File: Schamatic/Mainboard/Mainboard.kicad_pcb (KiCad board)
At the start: 2 copper layers, 45 x 130 mm, 277 parts, among them J1 CONN_01X02, J10 CONN_01X04, J2 CONN_01X02, J3 CONN_01X02, J4 CONN_01X02, J5 CONN_01X02, J6 CONN_02X05, J7 CONN_02X20, J8 CONN_01X02, J9 CONN_01X02, Q1 Q_NMOS_GDS, Q2 PSMN014-40YS, U1 LM2678-3.3V, U10 LTC2954, U2 LM2678-5V, U3 MC78M00, U4 LM5122, U5 UCC27611, U6 ACS781, U7 LSM6DS33, U8 STM32F031G6U6, U9 LTC2876, Y1 Resonator_Small

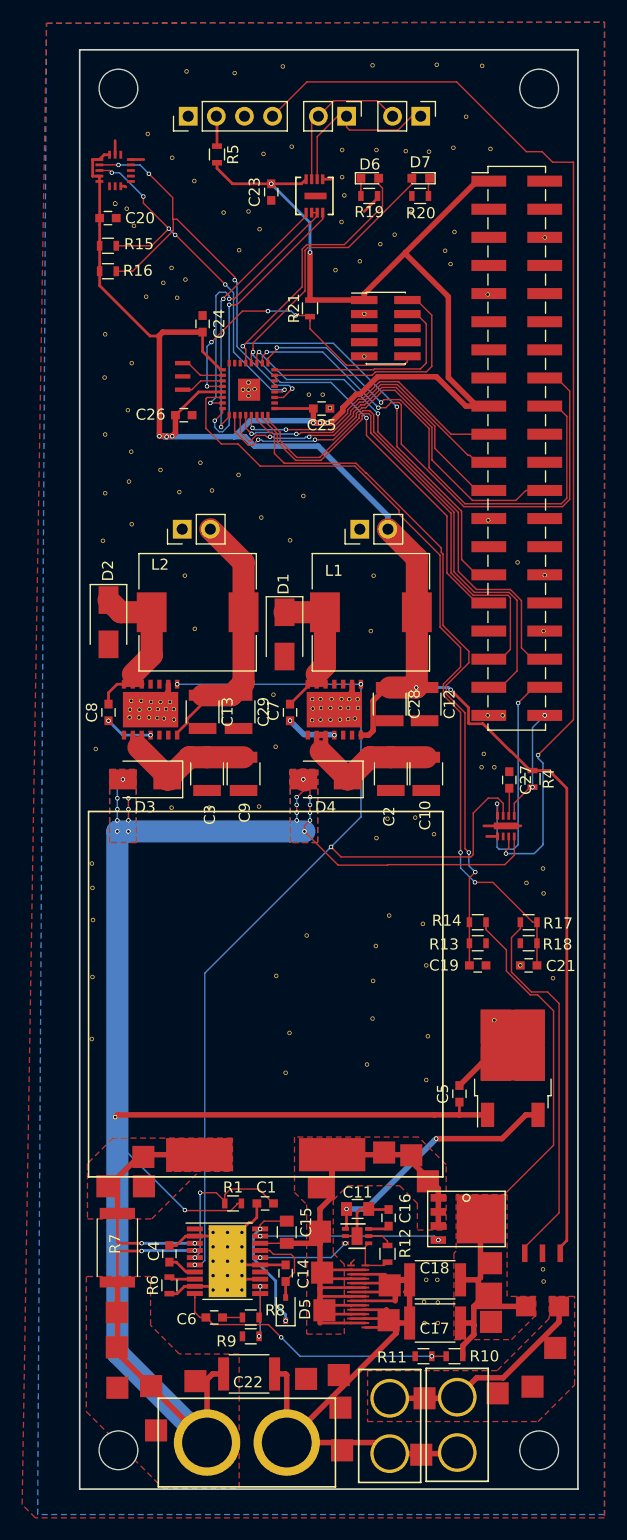
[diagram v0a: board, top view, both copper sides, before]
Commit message: changes
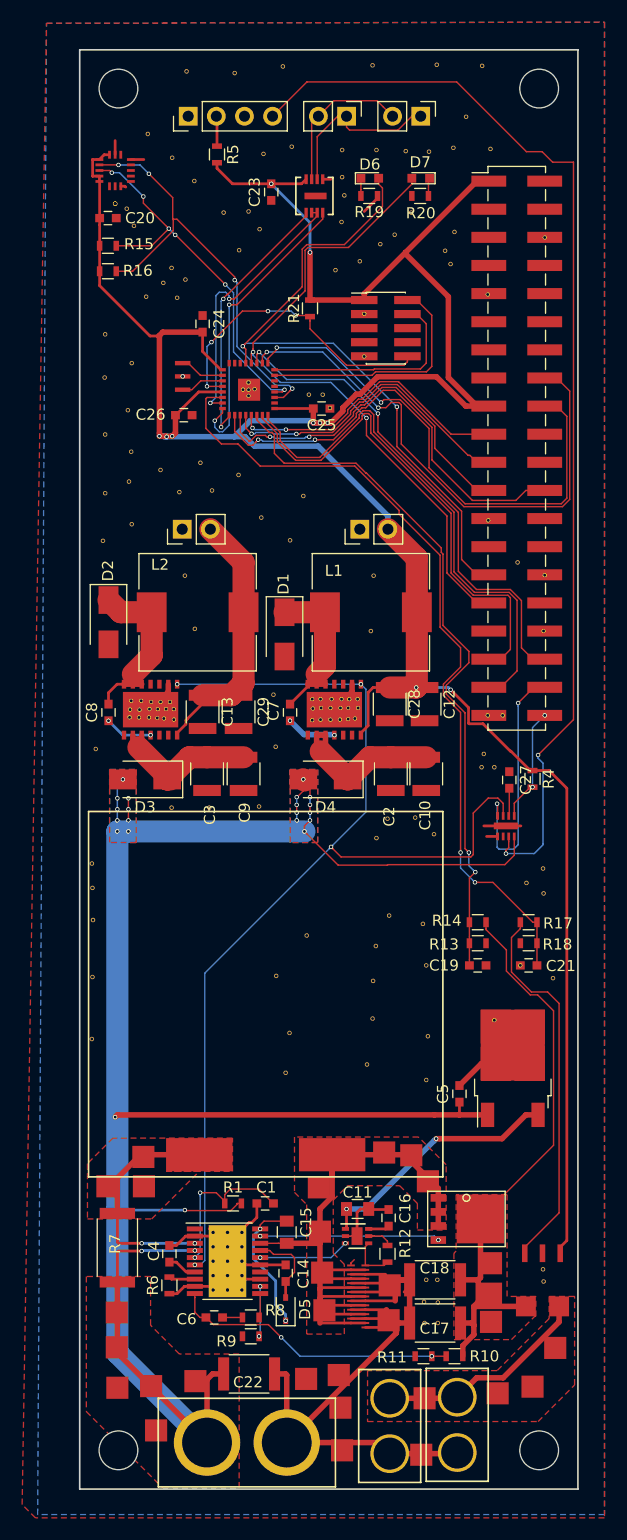
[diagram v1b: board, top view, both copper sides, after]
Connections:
- Y1 pad 2: (no net) -> Earth
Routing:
- net +BATT: track 200.3 -> 195.4 mm
- net 3.3V: track 250.1 -> 250.6 mm
- net Earth: vias 0 -> 1
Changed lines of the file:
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@@
 (kicad_pcb (version 4) (host pcbnew 4.0.6)
   (general
-    (links 0)
-    (no_connects 1)
-    (area 44.8 37.5 99.558572 172.600001)
+    (links 460)
+    (no_connects 2)
+    (area 49.924999 39.924999 95.075001 170.075001)
     (thickness 1.6)
     (drawings 4)
-    (tracks 1029)
+    (tracks 1034)
     (zones 0)
     (modules 277)
@@
     (47 F.CrtYd user)
     (48 B.Fab user)
-    (49 F.Fab user hide)
+    (49 F.Fab user)
   )
   (setup
-    (last_trace_width 0.13)
+    (last_trace_width 0.25)
     (user_trace_width 0.13)
     (user_trace_width 0.25)
@@
     (pad 1 smd rect (at 0 2.3 270) (size 0.4 1.4) (layers F.Cu F.Paste F.Mask)
       (net 50 "Net-(U8-Pad2)"))
-    (pad 2 smd rect (at 1.2 2.3 270) (size 0.4 1.4) (layers F.Cu F.Paste F.Mask))
+    (pad 2 smd rect (at 1.2 2.3 270) (size 0.4 1.4) (layers F.Cu F.Paste F.Mask)
+      (net 1 Earth))
     (pad 3 smd rect (at 2.4 2.3 270) (size 0.4 1.4) (layers F.Cu F.Paste F.Mask)
       (net 51 "Net-(U8-Pad3)"))
@@
   (gr_line (start 95 40) (end 95 170) (layer Edge.Cuts) (width 0.15))
   (gr_line (start 50 40) (end 95 40) (layer Edge.Cuts) (width 0.15))
+  (via (at 59.3 69.5) (size 0.4) (drill 0.25) (layers F.Cu B.Cu) (net 1))
   (segment (start 74.5 149.8) (end 74.5 149.58) (width 0.13) (layer F.Cu) (net 1))
   (segment (start 74.5 149.58) (end 74.8 149.28) (width 0.13) (layer F.Cu) (net 1))
@@
   (segment (start 58.725 149.5) (end 59.615 150.39) (width 0.25) (layer F.Cu) (net 3))
   (segment (start 59.615 150.39) (end 60.4 150.39) (width 0.25) (layer F.Cu) (net 3))
+  (segment (start 53.4 157.7) (end 53.4 144.75) (width 2) (layer B.Cu) (net 4))
+  (segment (start 53.4 144.75) (end 53.4 110.6) (width 2) (layer B.Cu) (net 4))
+  (segment (start 59.5 144.8) (end 53.45 144.8) (width 0.25) (layer B.Cu) (net 4))
+  (segment (start 53.45 144.8) (end 53.4 144.75) (width 0.25) (layer B.Cu) (net 4))
   (segment (start 88.4 113.6) (end 77.834602 113.6) (width 0.13) (layer F.Cu) (net 4))
   (segment (start 73.345001 113.645001) (end 70.499999 110.799999) (width 0.13) (layer F.Cu) (net 4))
@@
   (via (at 53.4 108.6) (size 0.4) (drill 0.25) (layers F.Cu B.Cu) (net 4))
   (via (at 53.4 109.6) (size 0.4) (drill 0.25) (layers F.Cu B.Cu) (net 4))
-  (segment (start 59.5 144.8) (end 53.2 138.5) (width 0.13) (layer B.Cu) (net 4))
-  (segment (start 53.2 138.5) (end 53.2 136.4) (width 0.13) (layer B.Cu) (net 4))
   (segment (start 64.22 144.28) (end 63.654999 144.845001) (width 0.13) (layer F.Cu) (net 4))
   (segment (start 63.654999 144.845001) (end 59.545001 144.845001) (width 0.13) (layer F.Cu) (net 4))
@@
   (segment (start 70.3 106) (end 70.2 105.9) (width 2) (layer F.Cu) (net 4))
   (via (at 70.3 110.6) (size 0.4) (drill 0.25) (layers F.Cu B.Cu) (net 4))
-  (segment (start 53.4 157.7) (end 53.4 110.6) (width 2) (layer B.Cu) (net 4))
   (via (at 53.4 110.6) (size 0.4) (drill 0.25) (layers F.Cu B.Cu) (net 4))
   (segment (start 61.5 165.8) (end 53.4 157.7) (width 2) (layer B.Cu) (net 4))
@@
   (segment (start 74.1 144.7) (end 74.1 146.4) (width 0.25) (layer F.Cu) (net 12))
   (segment (start 74.1 146.4) (end 74 146.5) (width 0.25) (layer F.Cu) (net 12))
+  (segment (start 78 97.6) (end 76.5 97.6) (width 0.25) (layer F.Cu) (net 13))
+  (segment (start 76.5 97.6) (end 76.05 98.05) (width 0.25) (layer F.Cu) (net 13))
+  (segment (start 76.05 98.05) (end 76.05 101.05) (width 0.25) (layer F.Cu) (net 13))
+  (segment (start 76.05 101.05) (end 75.4 101.7) (width 0.25) (layer F.Cu) (net 13))
+  (segment (start 75.4 101.7) (end 75.4 101.9) (width 0.25) (layer F.Cu) (net 13))
   (segment (start 85.119999 99.414978) (end 83.70502 97.999999) (width 0.25) (layer F.Cu) (net 13))
   (segment (start 88.9 103.35) (end 86.425001 100.875001) (width 0.25) (layer F.Cu) (net 13))
@@
   (segment (start 65.785161 75.799991) (end 64.93018 74.94501) (width 0.5) (layer B.Cu) (net 13))
   (segment (start 78 97.6) (end 77.7 97.6) (width 0.5) (layer F.Cu) (net 13))
-  (segment (start 77.7 97.6) (end 76.5 98.8) (width 0.5) (layer F.Cu) (net 13))
-  (segment (start 76.5 98.8) (end 76.5 101.5) (width 0.5) (layer F.Cu) (net 13))
-  (segment (start 76.5 101.5) (end 76.1 101.9) (width 0.5) (layer F.Cu) (net 13))
-  (segment (start 76.1 101.9) (end 75.4 101.9) (width 0.5) (layer F.Cu) (net 13))
   (segment (start 80.45 90.8) (end 80.45 85.91) (width 2) (layer F.Cu) (net 13))
   (segment (start 80.45 85.91) (end 77.84 83.3) (width 2) (layer F.Cu) (net 13))
@@
   (segment (start 75.7 62.035) (end 75.7 62.6) (width 0.5) (layer F.Cu) (net 13))
   (segment (start 88.025 72.18) (end 86.95 72.18) (width 0.5) (layer F.Cu) (net 13))
+  (segment (start 59.7 100.45) (end 59.594999 100.555001) (width 0.25) (layer F.Cu) (net 14))
+  (segment (start 59.594999 100.555001) (end 59.594999 100.905001) (width 0.25) (layer F.Cu) (net 14))
+  (segment (start 59.594999 100.905001) (end 58.8 101.7) (width 0.25) (layer F.Cu) (net 14))
   (segment (start 61.1 98.3) (end 61.1 99.05) (width 0.25) (layer F.Cu) (net 14))
   (segment (start 61.1 99.05) (end 59.7 100.45) (width 0.25) (layer F.Cu) (net 14))
-  (segment (start 59.7 100.8) (end 58.8 101.7) (width 0.25) (layer F.Cu) (net 14))
-  (segment (start 59.7 100.45) (end 59.7 100.8) (width 0.25) (layer F.Cu) (net 14))
   (segment (start 58.8 101.7) (end 58.8 101.9) (width 0.25) (layer F.Cu) (net 14))
   (segment (start 64.8 90.8) (end 64.8 86.3) (width 2) (layer F.Cu) (net 14))
@@
   (segment (start 89.25 108.05) (end 90.7 106.6) (width 0.13) (layer F.Cu) (net 56))
   (segment (start 90.7 106.6) (end 90.9 106.6) (width 0.13) (layer F.Cu) (net 56))
+  (segment (start 75.4 97.3) (end 75.85 97.75) (width 0.13) (layer B.Cu) (net 57))
+  (segment (start 75.85 97.75) (end 75.85 108.85) (width 0.13) (layer B.Cu) (net 57))
+  (segment (start 75.85 108.85) (end 72.899999 111.800001) (width 0.13) (layer B.Cu) (net 57))
+  (segment (start 72.899999 111.800001) (end 72.7 112) (width 0.13) (layer B.Cu) (net 57))
   (segment (start 85.545002 112.689602) (end 85.334605 112.899999) (width 0.13) (layer F.Cu) (net 57))
-  (segment (start 75.4 97.3) (end 75.4 109.3) (width 0.13) (layer B.Cu) (net 57))
   (segment (start 87.774206 107.589602) (end 86.895002 107.589602) (width 0.13) (layer F.Cu) (net 57))
   (segment (start 88.25 108.065396) (end 87.774206 107.589602) (width 0.13) (layer F.Cu) (net 57))
-  (segment (start 72.899999 111.800001) (end 72.7 112) (width 0.13) (layer B.Cu) (net 57))
-  (segment (start 75.4 109.3) (end 72.899999 111.800001) (width 0.13) (layer B.Cu) (net 57))
   (segment (start 88.25 109.2) (end 88.25 108.065396) (width 0.13) (layer F.Cu) (net 57))
   (segment (start 72.500001 112.199999) (end 72.7 112) (width 0.13) (layer B.Cu) (net 57))
